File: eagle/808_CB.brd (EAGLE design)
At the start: 100 x 80 mm, 54 parts, among them IC1 4584N, IC4 TL072P, Q1 2N3904, Q2 2N3904, Q3 2N3904, Q8 2N3906

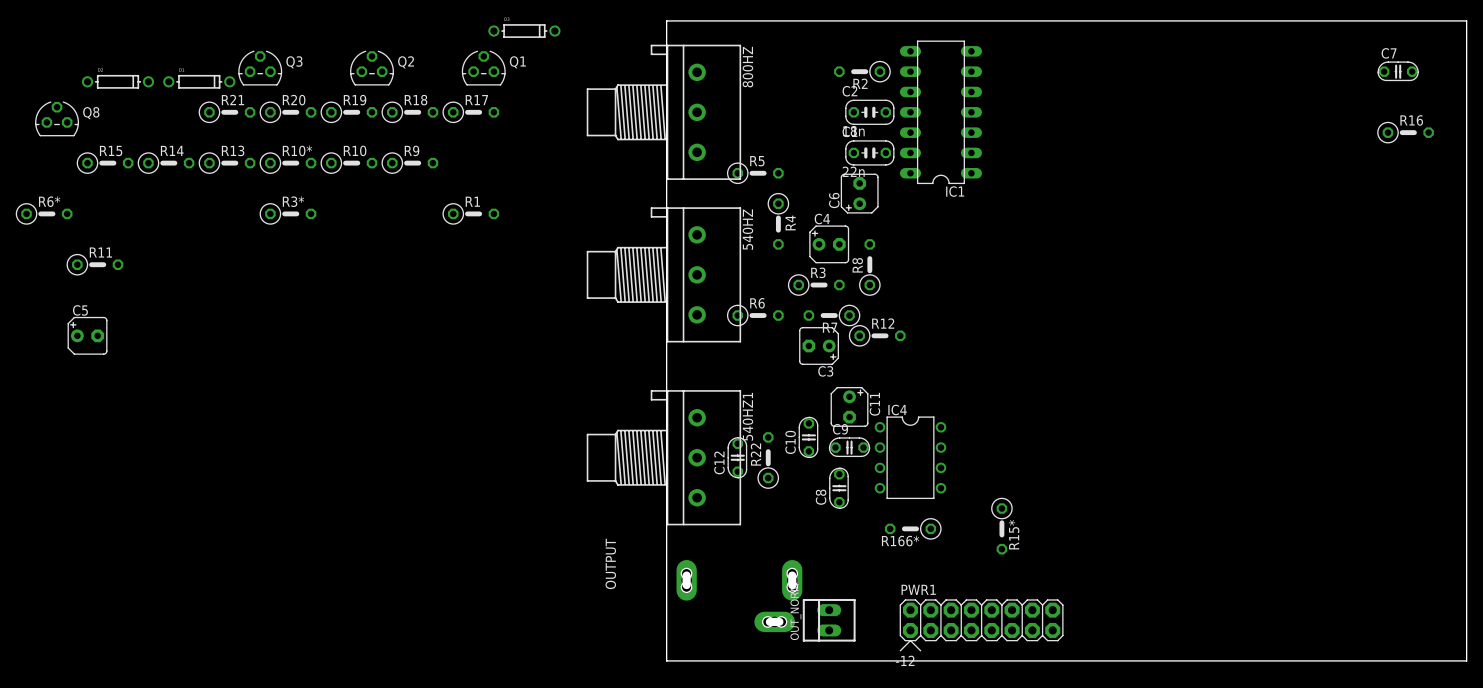
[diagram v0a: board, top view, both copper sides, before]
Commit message: starting board part by part
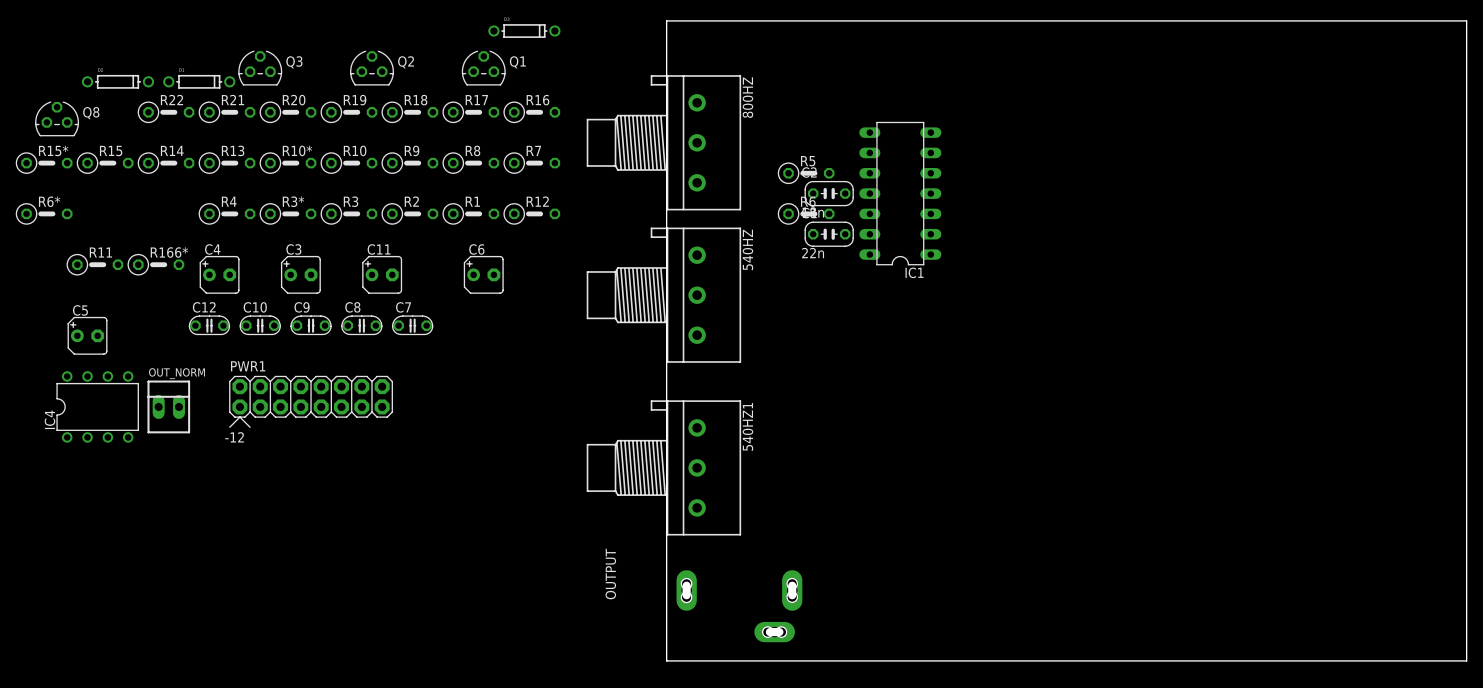
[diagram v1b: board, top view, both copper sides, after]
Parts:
- moved R15* 127.8 mm to (-77.5, 62.2), turned to 0 degrees
- moved C7 127.2 mm to (-31.8, 41.9)
- moved R16 109.2 mm to (-16.5, 68.6)
- moved IC4 101.8 mm to (-71.1, 31.8), turned to 0 degrees
- moved R166* 99.6 mm to (-63.5, 49.5), turned to 0 degrees
- moved PWR1 88.4 mm to (-47.0, 33.0)
- moved OUT_NORM 86.8 mm to (-62.2, 31.8), turned to 0 degrees
- moved R22 86.5 mm to (-62.2, 68.6), turned to 0 degrees
- moved C4 76.3 mm to (-55.9, 48.3)
- moved C10 70.0 mm to (-50.8, 41.9), turned to 0 degrees
- moved C9 69.0 mm to (-44.5, 41.9)
- moved R4 68.6 mm to (-54.6, 55.9), turned to 0 degrees
- moved C12 68.1 mm to (-57.1, 41.9), turned to 0 degrees
- moved C3 65.4 mm to (-45.7, 48.3), turned to 0 degrees
- moved C8 63.1 mm to (-38.1, 41.9), turned to 0 degrees
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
